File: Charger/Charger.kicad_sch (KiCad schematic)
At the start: 15 parts, among them SW2 SW_Push, U1 ATmega328-A, Y1 20MHz

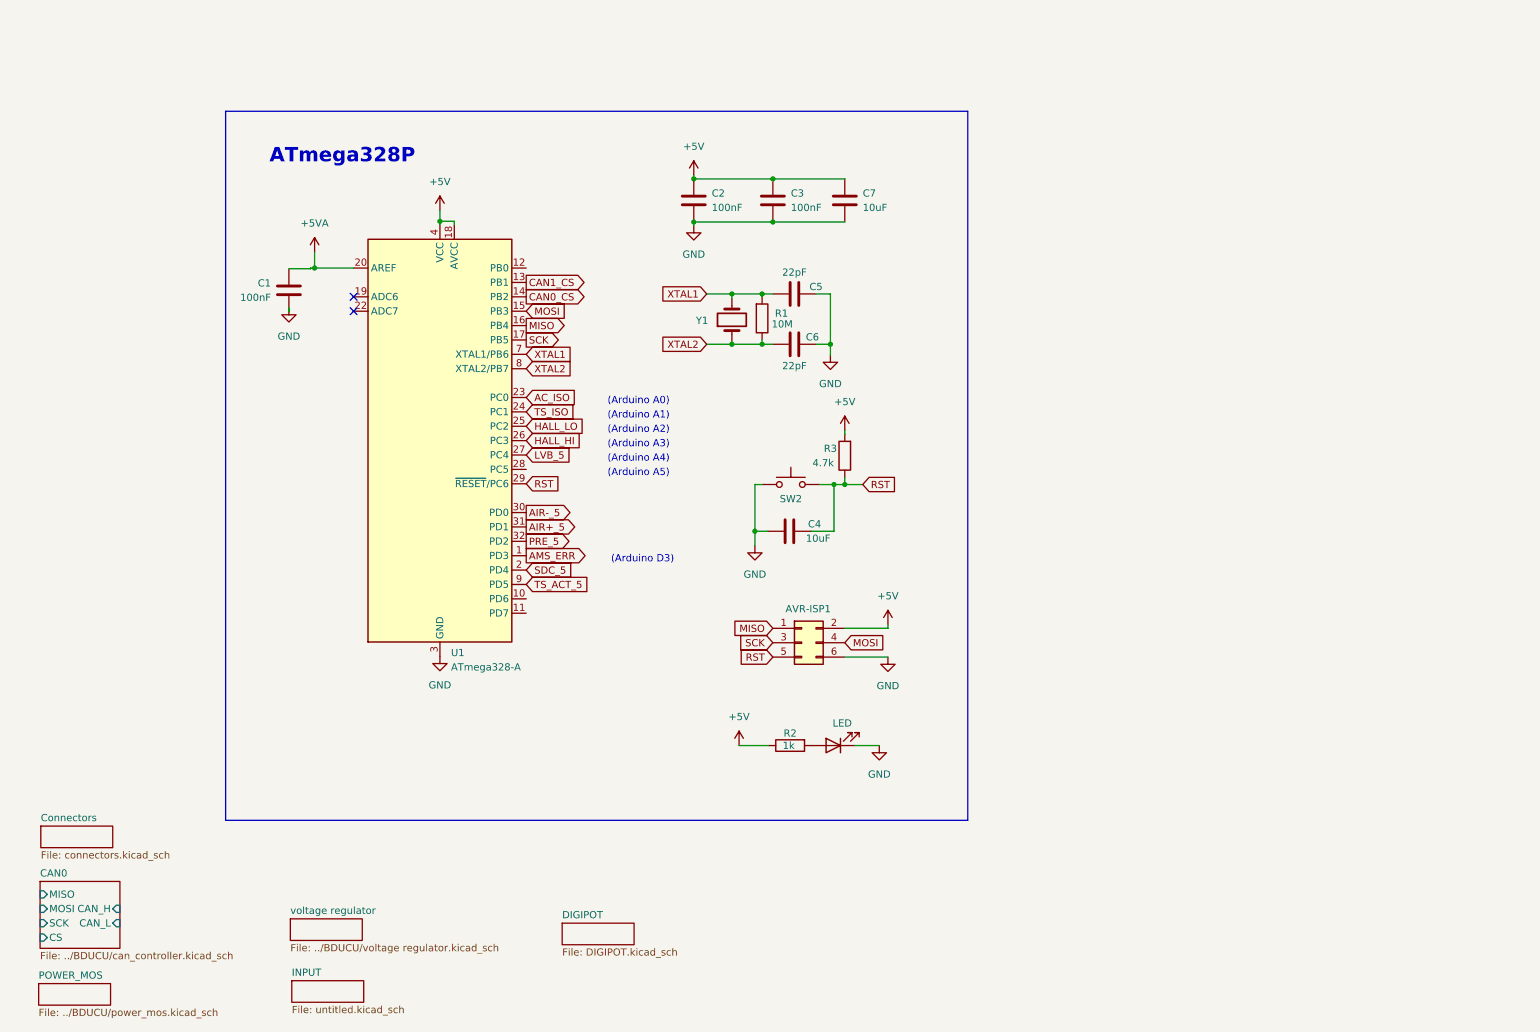
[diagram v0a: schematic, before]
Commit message: funny stuffs
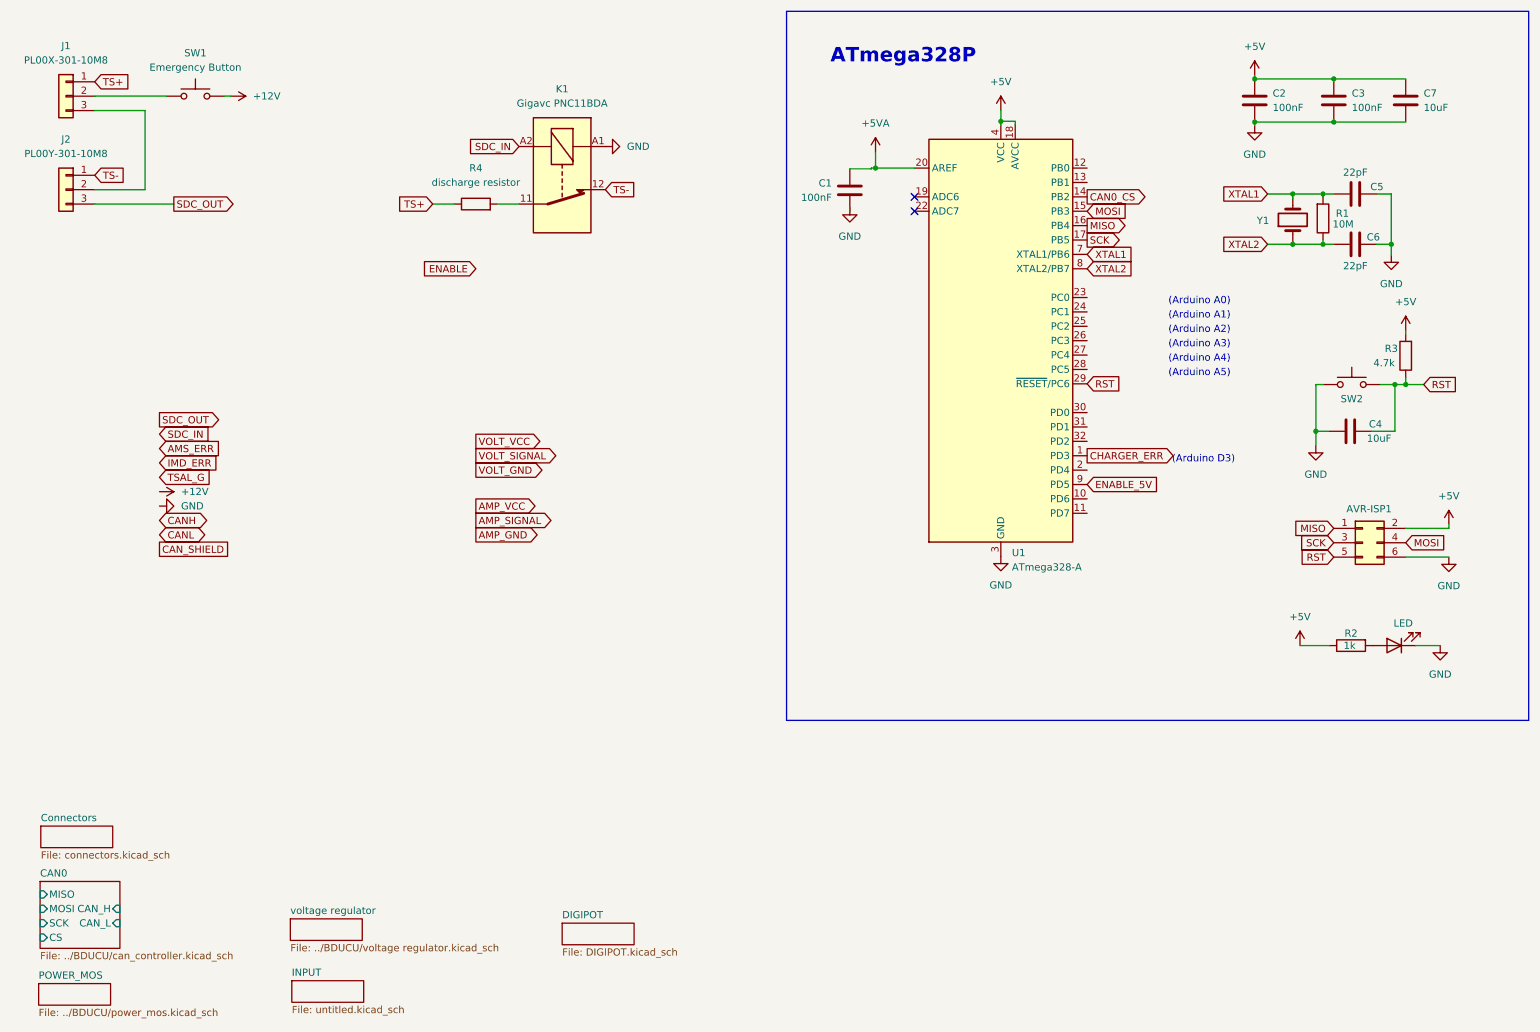
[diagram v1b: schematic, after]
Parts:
- added J1: PL00X-301-10M8, symbol Connector_Generic:Conn_01x03
- added J2: PL00Y-301-10M8, symbol Connector_Generic:Conn_01x03
- added K1: Gigavc PNC11BDA, symbol Relay:Relay_SPST-NC
- added R4: discharge resistor, symbol Device:R
- added SW1: Emergency Button, symbol Switch:SW_Push
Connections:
- net AMS_ERR: no longer U1.1 (PD3)
- net GND: now also K1.A1
- net AC_ISO: no longer names the net of U1.23 (PC0)
- net AIR+_5: no longer names the net of U1.31 (PD1)
- net AIR-_5: no longer names the net of U1.30 (PD0)
- net CAN1_CS: no longer names the net of U1.13 (PB1)
- net HALL_HI: no longer names the net of U1.26 (PC3)
- net HALL_LO: no longer names the net of U1.25 (PC2)
- net LVB_5: no longer names the net of U1.27 (PC4)
- net PRE_5: no longer names the net of U1.32 (PD2)
- net SDC_5: no longer names the net of U1.2 (PD4)
- net TS_ACT_5 renamed ENABLE_5V
- net TS_ISO: no longer names the net of U1.24 (PC1)
- new net: J1.2 (Pin_2), SW1.1
- new net: J1.3 (Pin_3), J2.2 (Pin_2)
- new net: K1.11, R4.2
- new net +12V: SW1.2
- new net CHARGER_ERR: U1.1 (PD3)
- new net SDC_IN: K1.A2
- new net SDC_OUT: J2.3 (Pin_3)
- new net TS+: J1.1 (Pin_1), R4.1
- new net TS-: J2.1 (Pin_1), K1.12
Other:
- moved on the sheet: AVR-ISP1, C1, C2, C3, C4, C5, C6, C7, R1, R2, R3, SW2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
